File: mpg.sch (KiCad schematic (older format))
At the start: 40 parts, among them J1 Conn_01x04_Male, J2 DB25_Male_MountingHoles, J3 Conn_01x03_Male, J4 Screw_Terminal_01x02, J5 Screw_Terminal_01x03, J6 Screw_Terminal_01x03, K1 G5LE-1, Q1 BC847, Q2 BC847, Q3 BC847, Q4 BC847, Q5 BC847, SW1 SW_Push, U1 LD2981ABU33TR, U2 STM32G031F4Px, U3 SP3485CN

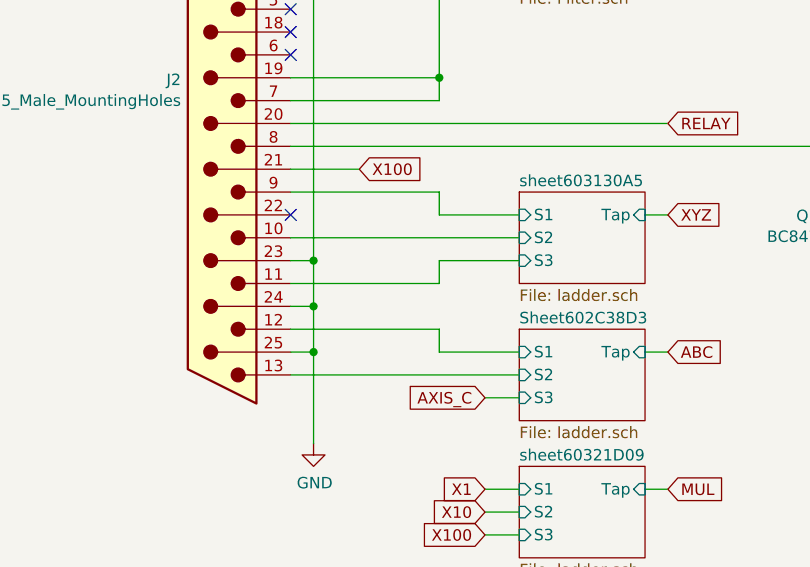
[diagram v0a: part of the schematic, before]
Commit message: Better layout.
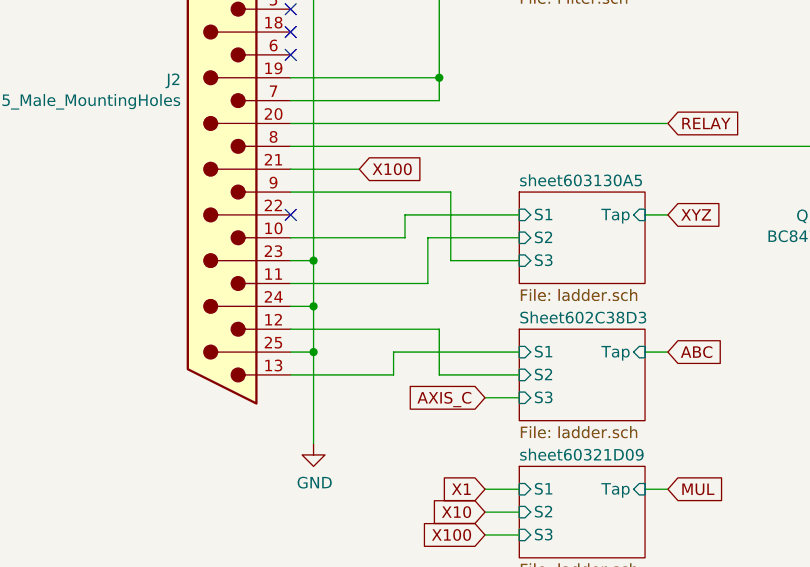
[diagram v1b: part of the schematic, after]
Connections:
- net Sheet602C38D3/S1: now also J2.13; no longer J2.12
- net Sheet602C38D3/S2: now also J2.12; no longer J2.13
- net sheet603130A5/S1: now also J2.10; no longer J2.9
- net sheet603130A5/S2: now also J2.11; no longer J2.10
- net sheet603130A5/S3: now also J2.9; no longer J2.11
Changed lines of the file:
@@
 	3750 4850 3900 4850
 Wire Wire Line
-	2900 4750 3900 4750
-Wire Wire Line
 	2900 4550 3550 4550
-Wire Wire Line
-	3550 4550 3550 4650
-Wire Wire Line
-	3550 4650 3900 4650
 $Sheet
 S 3900 3950 550  400
@@
 $EndSheet
 Wire Wire Line
-	3550 4050 3900 4050
-Wire Wire Line
-	2900 4150 3900 4150
-Wire Wire Line
-	3550 4350 3550 4250
-Wire Wire Line
-	2900 4350 3550 4350
-Wire Wire Line
-	3550 4250 3900 4250
-Wire Wire Line
-	3550 3950 3550 4050
-Wire Wire Line
-	2900 3950 3550 3950
+	2900 4350 3500 4350
 $Sheet
 S 3900 5150 550  400
@@
 	1    0    0    -1
 $EndComp
+Wire Wire Line
+	3550 4750 3900 4750
+Wire Wire Line
+	3550 4550 3550 4750
+Wire Wire Line
+	2900 4750 3350 4750
+Wire Wire Line
+	3350 4750 3350 4650
+Wire Wire Line
+	3350 4650 3900 4650
+Wire Wire Line
+	3600 4250 3900 4250
+Wire Wire Line
+	2900 3950 3600 3950
+Wire Wire Line
+	2900 4150 3400 4150
+Wire Wire Line
+	3600 3950 3600 4250
+Wire Wire Line
+	3400 4050 3900 4050
+Wire Wire Line
+	3400 4050 3400 4150
+Wire Wire Line
+	3500 4150 3900 4150
+Wire Wire Line
+	3500 4150 3500 4350
 $EndSCHEMATC
